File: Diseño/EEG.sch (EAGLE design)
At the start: 32 parts, among them IC1 REF2033AIDDCT, IC2 MCP73831T-2ACI_OT, IC3 LP38692MP-3.3_NOPB, X1 MINI-USB_4P-85-32004-40X

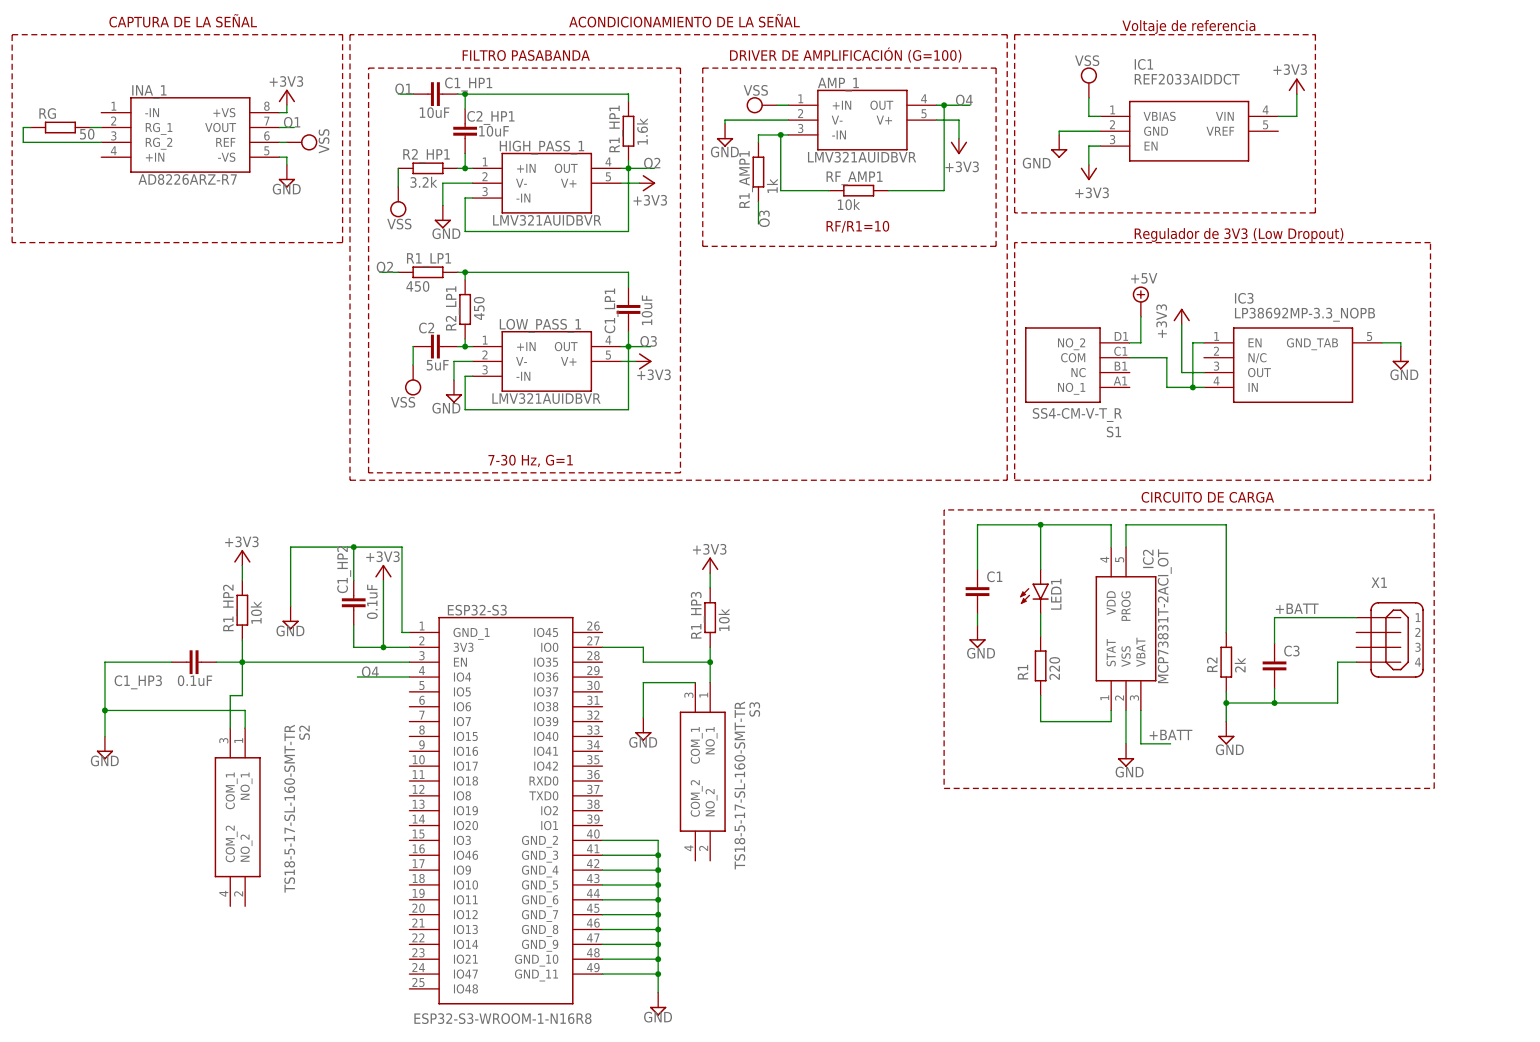
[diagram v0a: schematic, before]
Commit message: correcciones
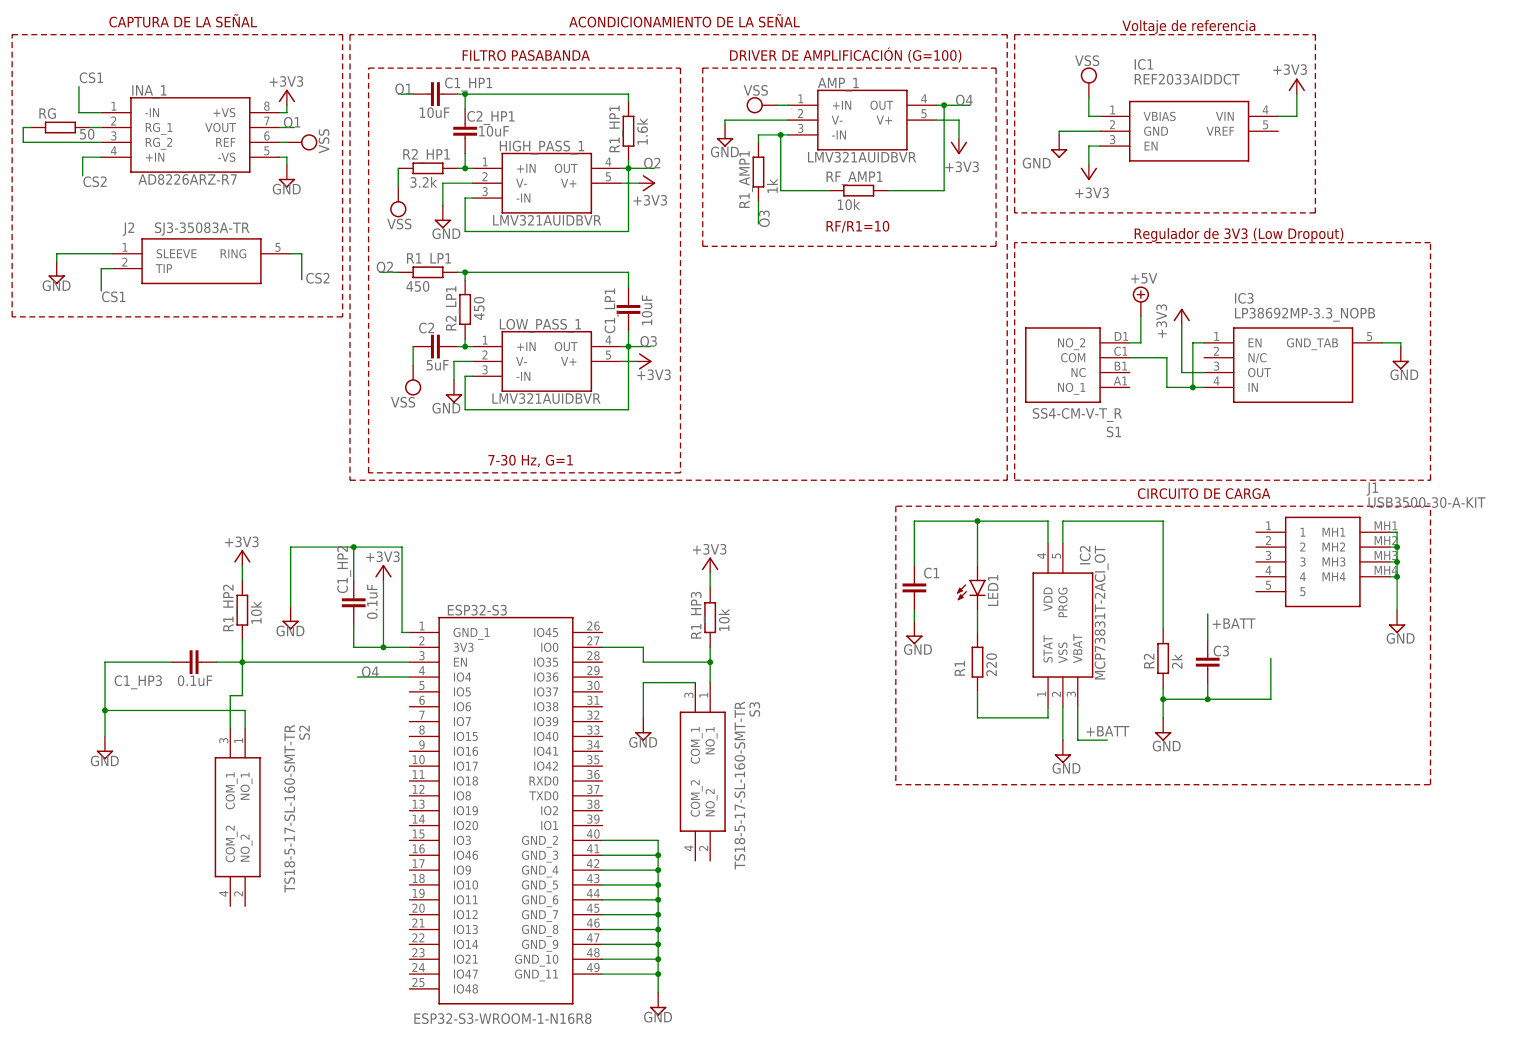
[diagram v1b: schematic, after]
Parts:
- removed X1: MINI-USB_4P-85-32004-40X, con-cypressindustries:MINI-USB_4P-85-32004-40X
- added J1: USB3500-30-A-KIT, USB3500-30-A-KIT:USB3500-30-A-KIT
- added J2: SJ3-35083A-TR, SJ3-35083A-TR:SJ3-35083A-TR
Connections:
- new net CS1: INA_1.-IN, J2.TIP
- new net CS2: INA_1.+IN, J2.RING
- net +BATT: no longer X1.1
- net GND: now also J1.MH1, J1.MH2, J1.MH3, J1.MH4, J2.SLEEVE; no longer X1.4
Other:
- moved on the sheet: C1, C3, IC2, LED1, R1, R2
